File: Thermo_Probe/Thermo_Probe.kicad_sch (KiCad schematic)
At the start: 20 parts, among them J1 Power, J2 Digital/PWM, J3 Analog, J4 Digital/PWM, J5 GYRO_CONN, J6 Connector Display, J7 CONN_TEMP, SW1 SW_SPST, SW2 SW_SPST, SW3 SW_SPST, SW4 SW_SPST, SW5 SW_SPST

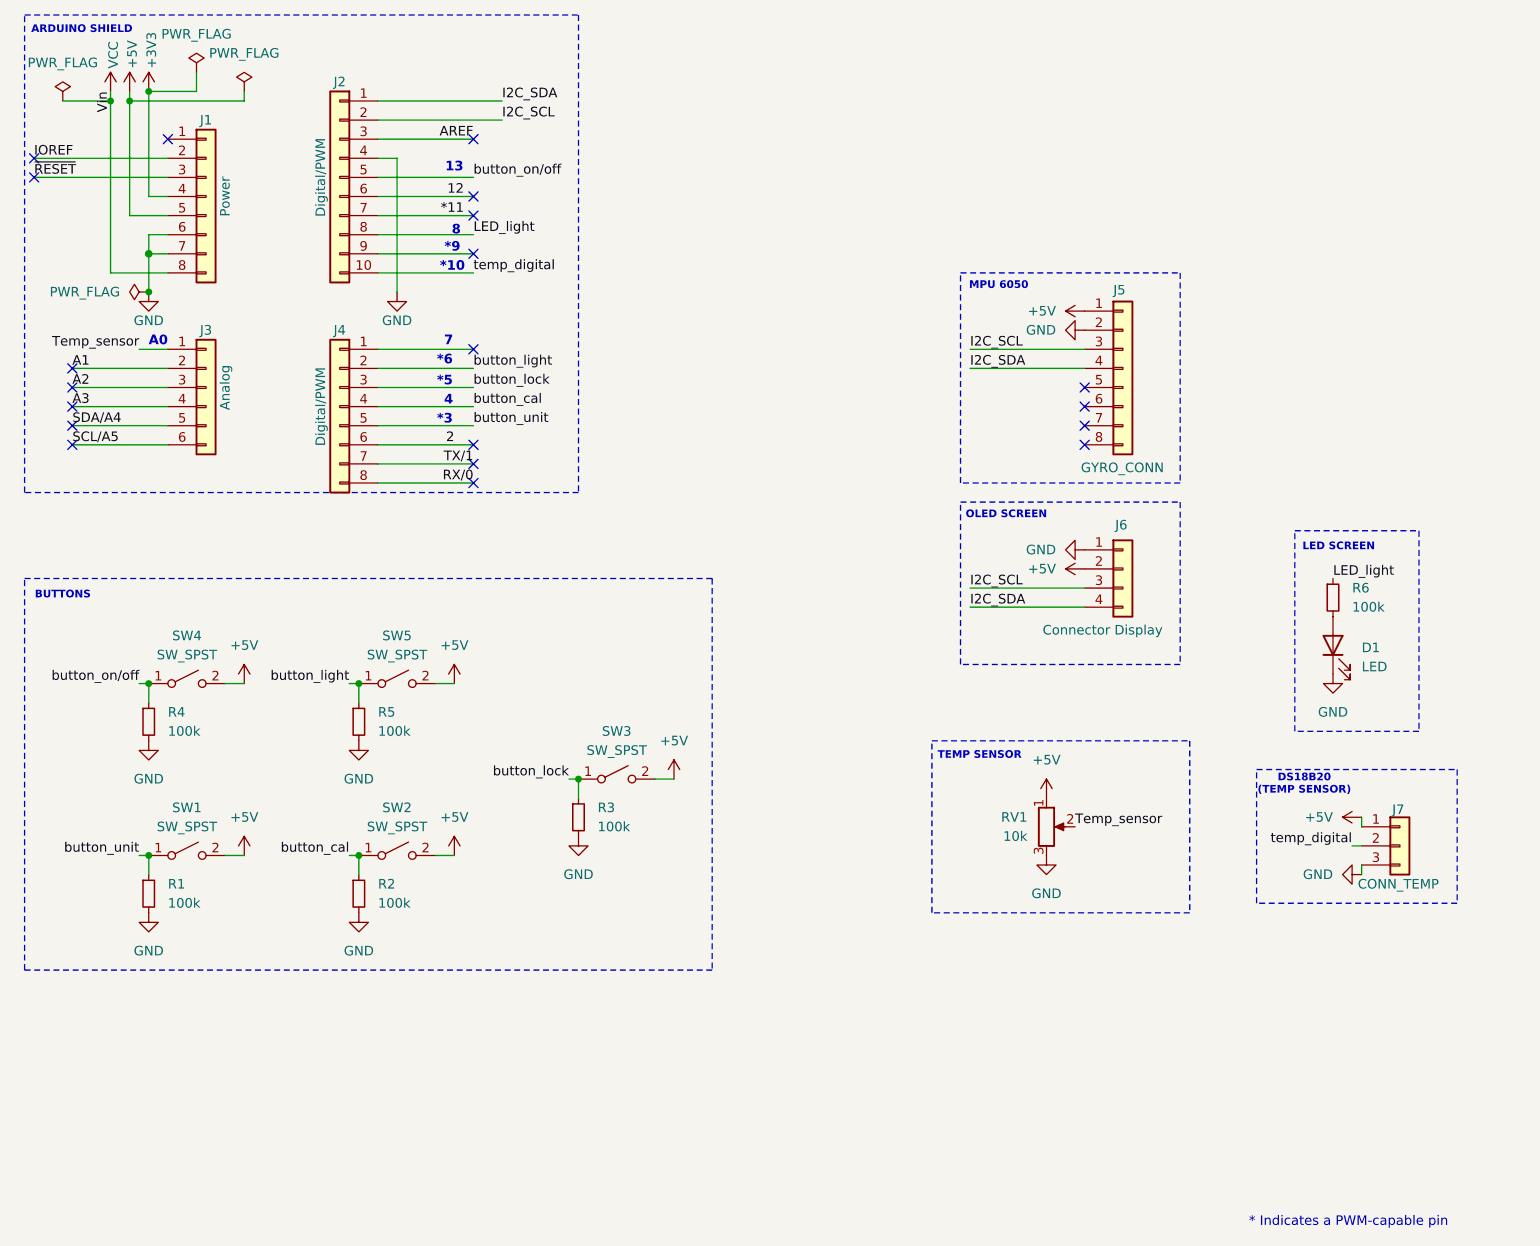
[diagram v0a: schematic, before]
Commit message: Probe
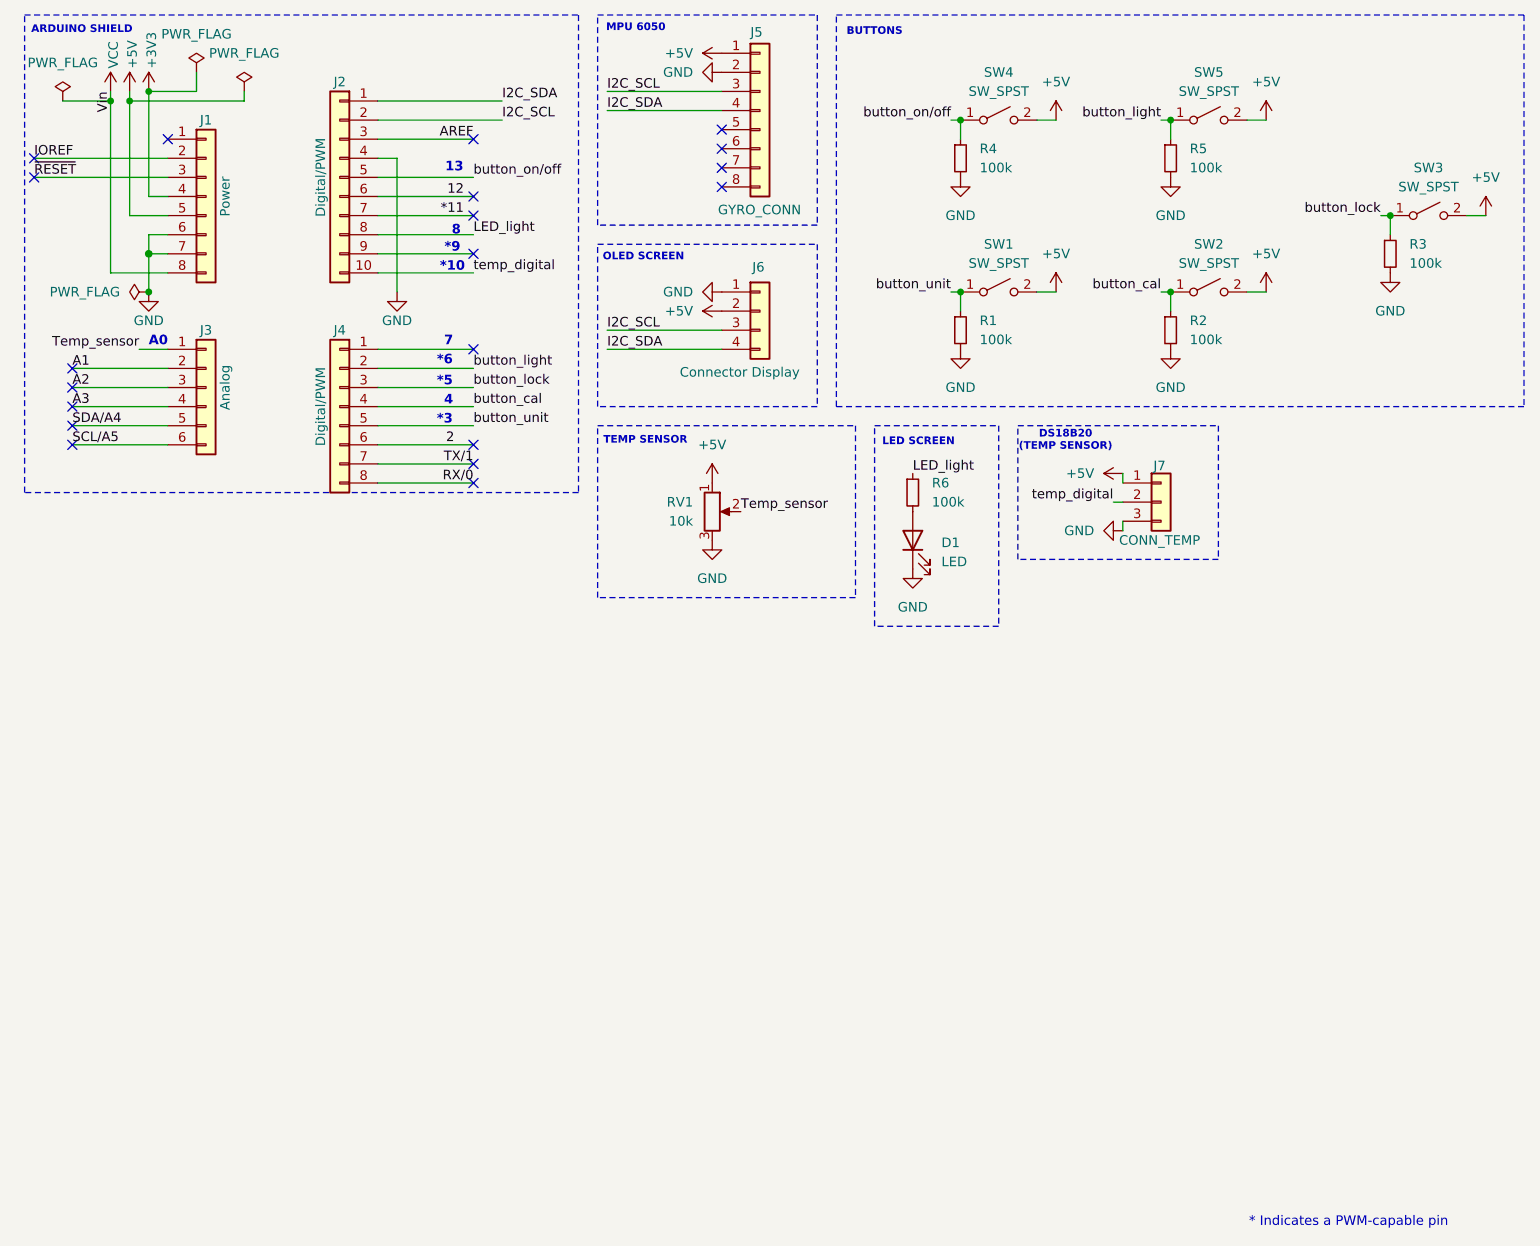
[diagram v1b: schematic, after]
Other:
- moved on the sheet: D1, J5, J6, J7, R1, R2, R3, R4, R5, R6, RV1, SW1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
